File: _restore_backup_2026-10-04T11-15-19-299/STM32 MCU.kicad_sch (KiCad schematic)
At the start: 21 parts, among them SW3 SW_Push, SW4 SW_Push, U2 STM32G474RETx, Y1 Crystal

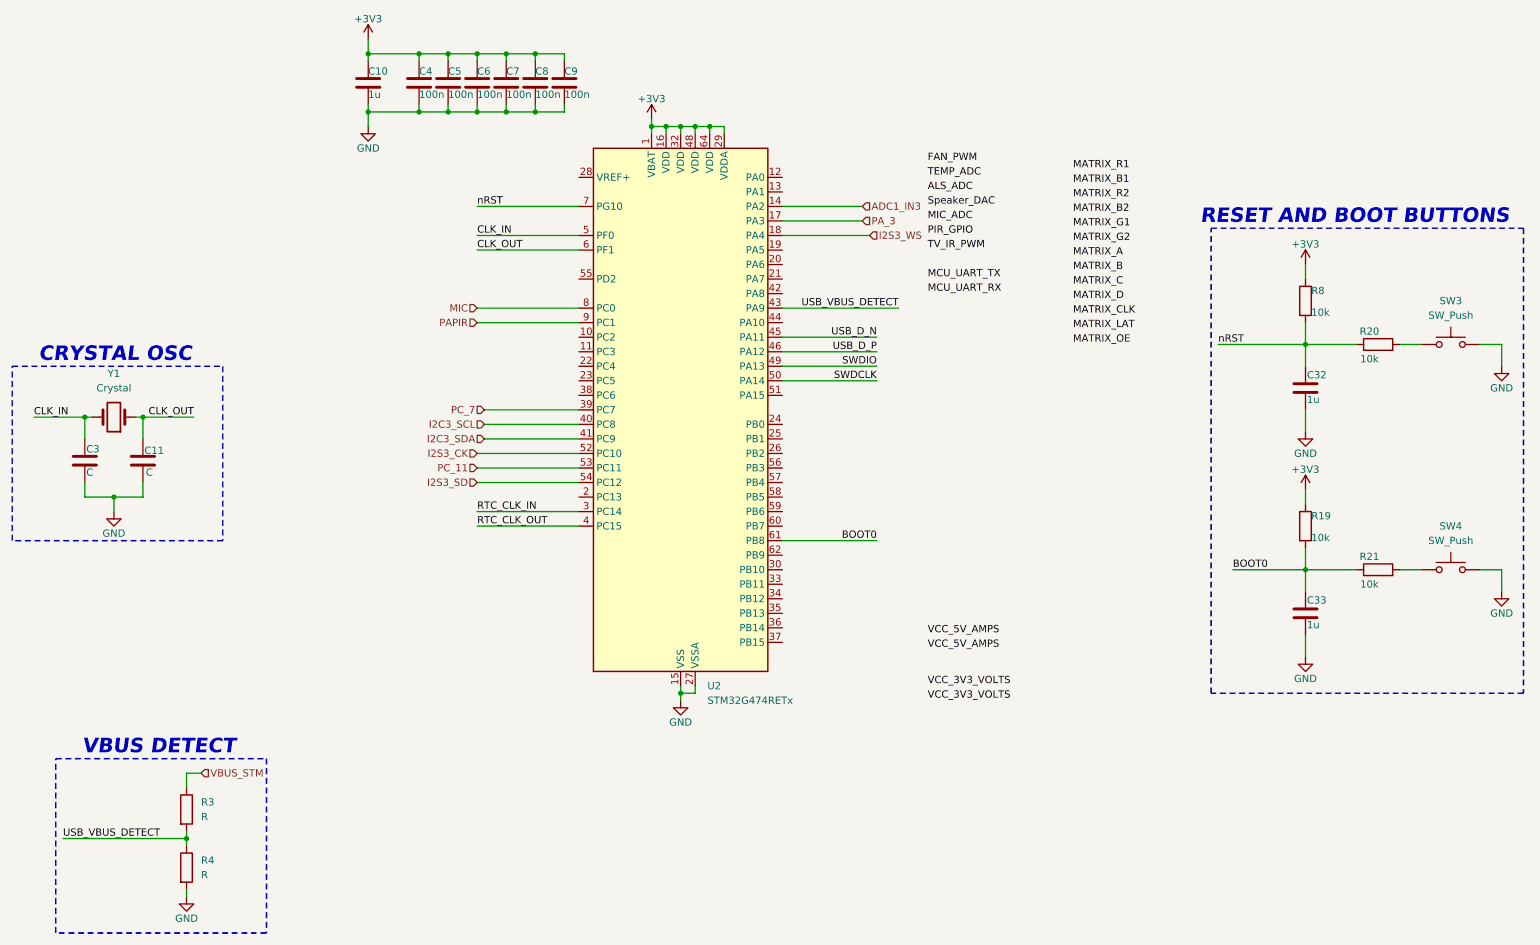
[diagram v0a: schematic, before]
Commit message: Schematic work 10/4
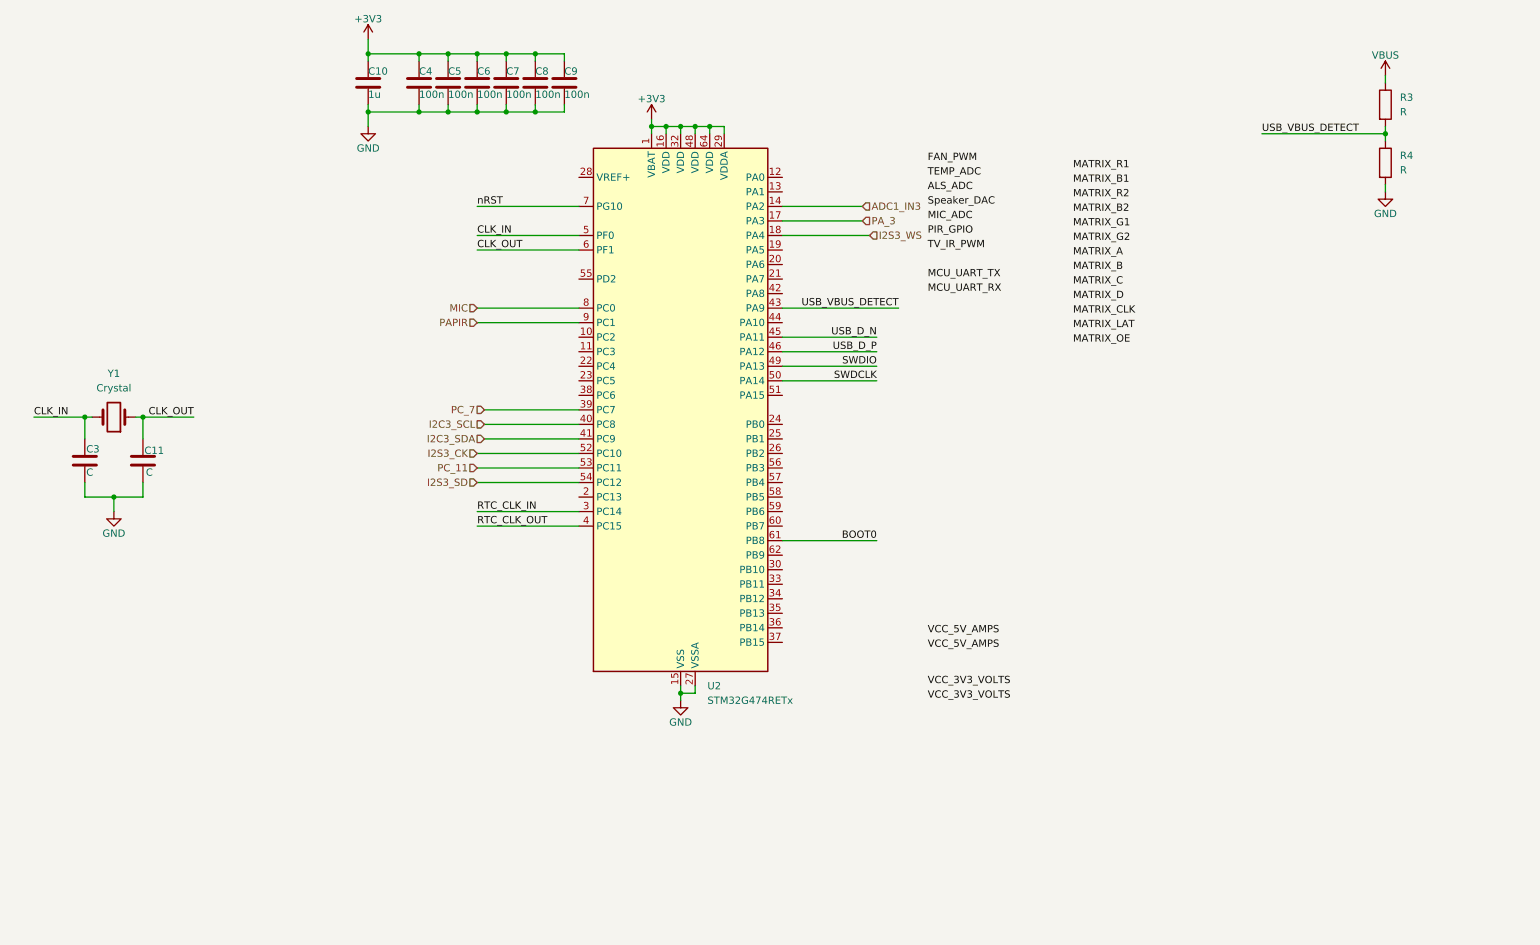
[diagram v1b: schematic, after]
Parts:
- removed C32, C33: 1u, symbol Device:C
- removed R19, R20, R21, R8: 10k, Package_DIP:DIP-8_W7.62mm, symbol Device:R
- removed SW3, SW4: SW_Push, Package_DIP:DIP-8_W7.62mm, symbol Switch:SW_Push
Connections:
- net VBUS_STM renamed VBUS
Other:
- note removed: "CRYSTAL OSC"
- note removed: "RESET AND BOOT BUTTONS"
- note removed: "VBUS DETECT"
- moved on the sheet: R3, R4
